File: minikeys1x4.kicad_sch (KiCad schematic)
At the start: 15 parts

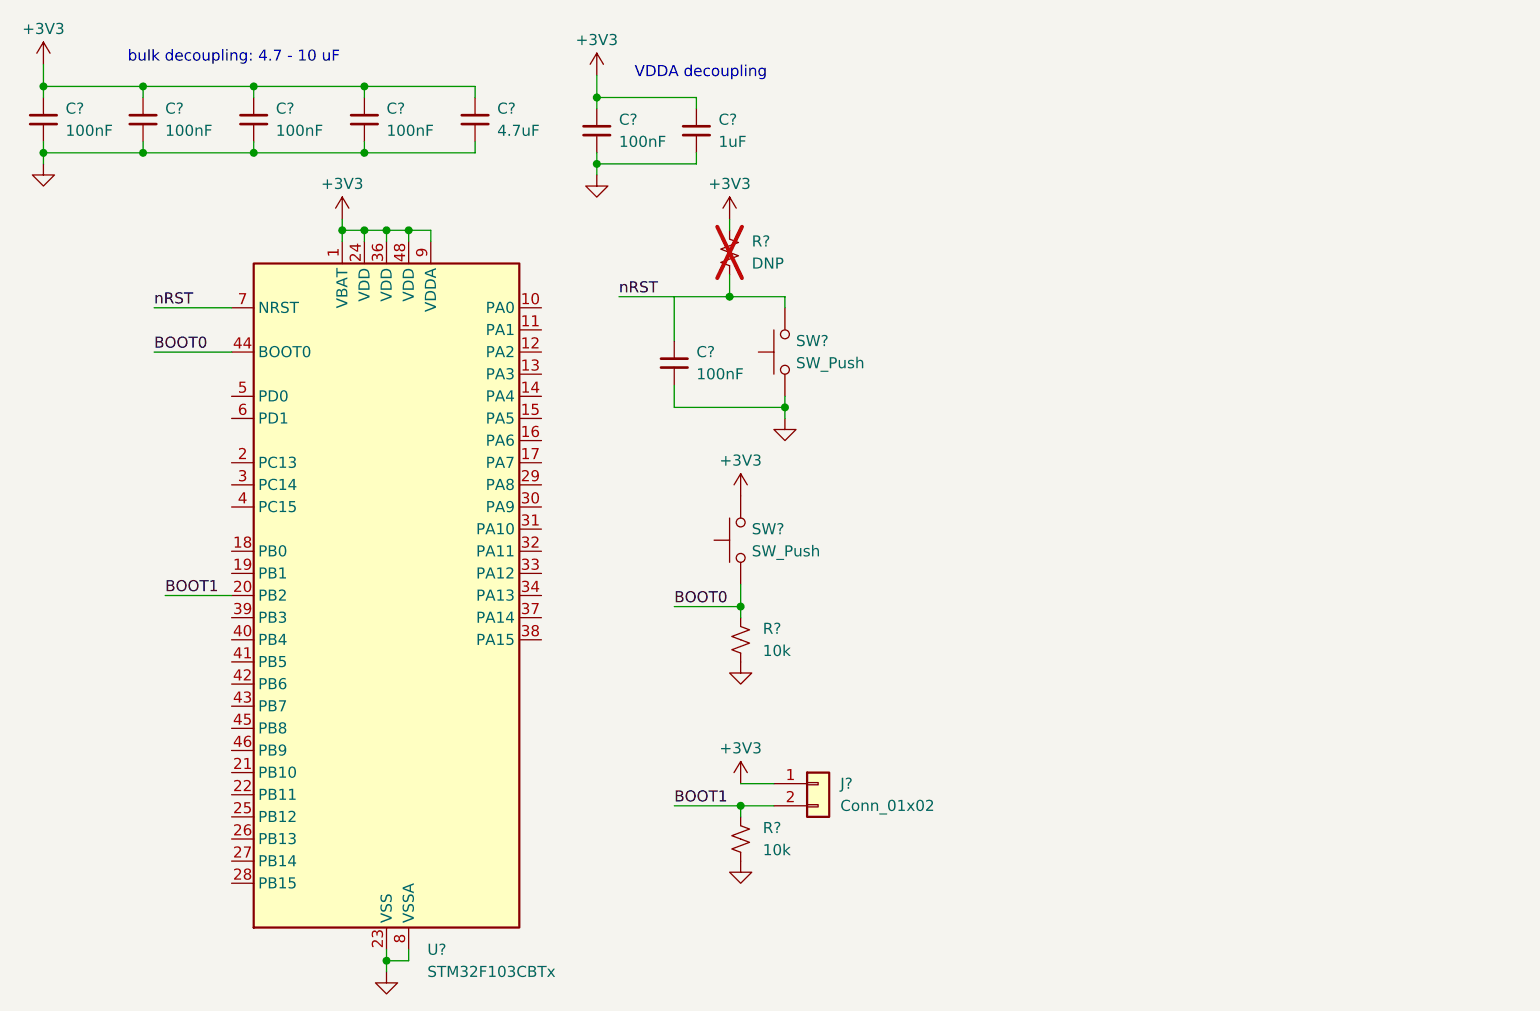
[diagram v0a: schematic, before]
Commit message: add placeholder keys, xtals, LED, debug
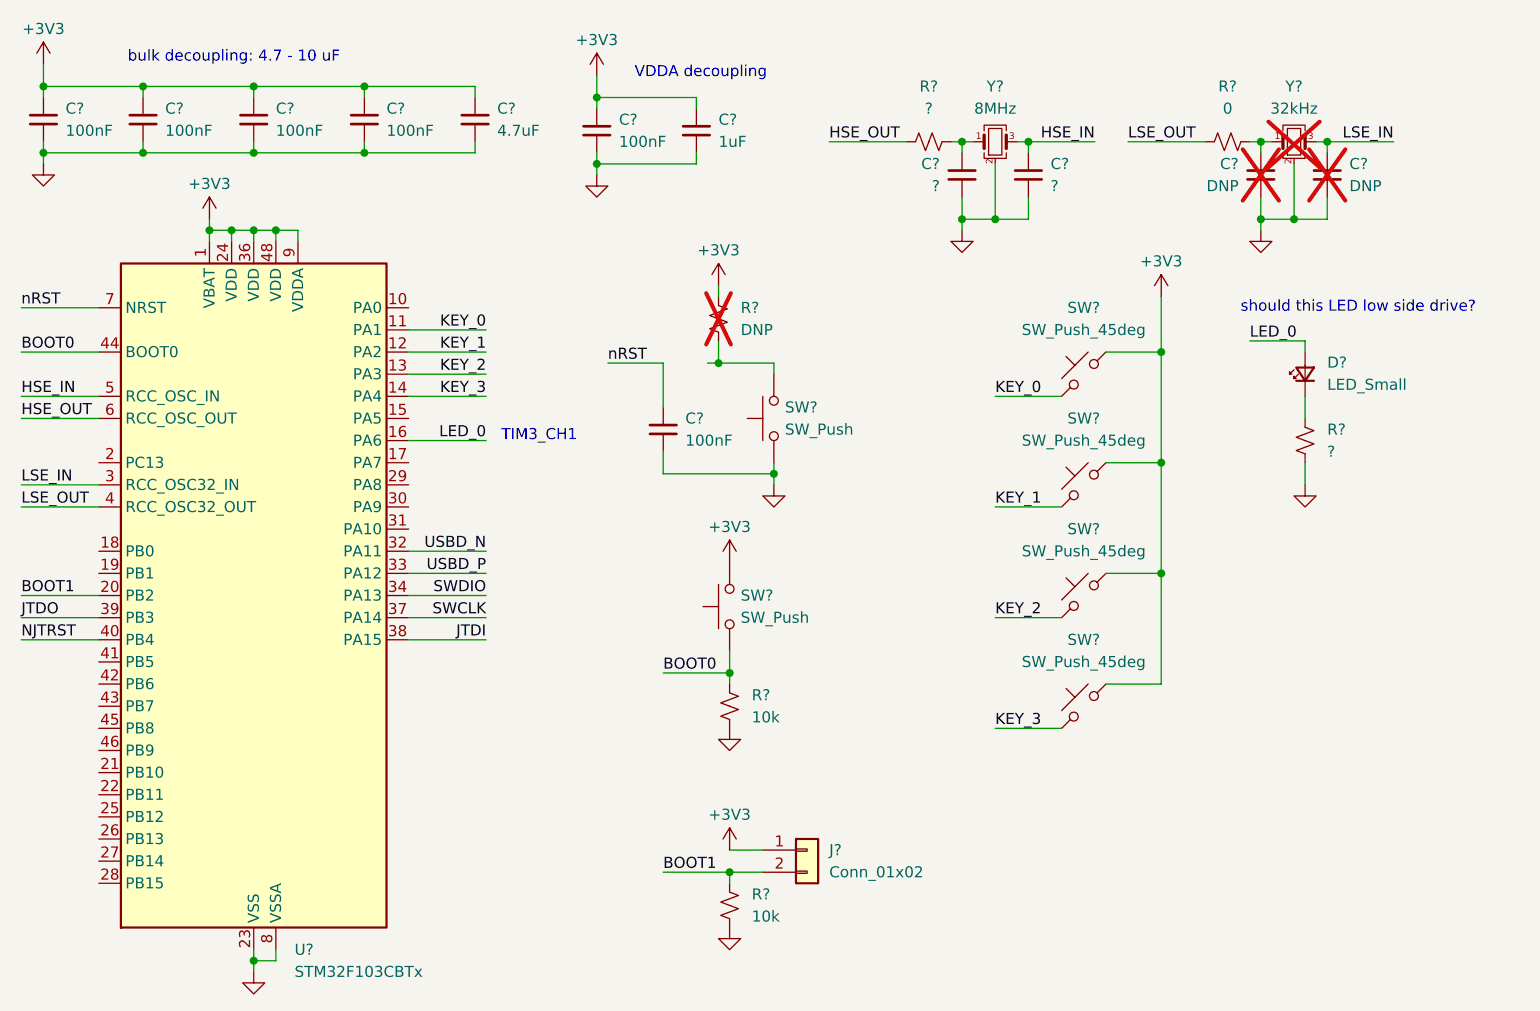
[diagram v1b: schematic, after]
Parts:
- added C? (x2): DNP, symbol Device:C_Small
- added C? (x2): ?, symbol Device:C_Small
- added D?: LED_Small, symbol Device:LED_Small
- added R? (x2): ?, symbol Device:R_Small_US
- added R?: 0, symbol Device:R_Small_US
- added SW? (x4): SW_Push_45deg, symbol Switch:SW_Push_45deg
- added Y?: 32kHz, symbol Device:Crystal_GND24_Small
- added Y?: 8MHz, symbol Device:Crystal_GND24_Small
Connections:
- net +3V3: now also SW?.1, SW?.1, SW?.1, SW?.1
- net GND: now also C?.2, C?.2, C?.2, C?.2, R?.2, Y?.2 (G), Y?.2 (G), Y?.4 (G), Y?.4 (G)
- net nRST: now also C?.1; no longer R?.2, SW?.1
- net KEY_0: now reaches U?.11 (PA1)
- net KEY_0: now also SW?.2
- net KEY_1: now reaches U?.12 (PA2)
- net KEY_1: now also SW?.2
- net KEY_2: now reaches U?.13 (PA3)
- net KEY_2: now also SW?.2
- net KEY_3: now reaches U?.14 (PA4)
- net KEY_3: now also SW?.2
- net LED_0: now reaches U?.16 (PA6)
- net LED_0: now also D?.2 (A)
- net LSE_IN: now reaches U?.3 (PC14)
- net LSE_IN: now also C?.1, Y?.3
- net USBD_N: now reaches U?.32 (PA11)
- net USBD_P: now reaches U?.33 (PA12)
- net SWDIO: now reaches U?.34 (PA13)
- net SWCLK: now reaches U?.37 (PA14)
- net JTDI: now reaches U?.38 (PA15)
- net JTDO: now reaches U?.39 (PB3)
- net LSE_OUT: now reaches U?.4 (PC15)
- net LSE_OUT: now also R?.1
- net NJTRST: now reaches U?.40 (PB4)
- net HSE_IN: now reaches U?.5 (PD0)
- net HSE_IN: now also C?.1, Y?.3
- net HSE_OUT: now reaches U?.6 (PD1)
- net HSE_OUT: now also R?.1
- new net: R?.2, SW?.1
- new net: C?.1, R?.2, Y?.1 (x2)
- new net: D?.1 (K), R?.1
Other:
- note added: "TIM3_CH1"
- note added: "should this LED low side drive?"
- moved on the sheet: C?, J?, R?, SW?, U?
